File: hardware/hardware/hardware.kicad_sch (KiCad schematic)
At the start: 31 parts, among them J1 POWER, J2 SENSOR, Q1 BC547, Q2 NPN, Q3 NPN, Q4 NPN, Q5 NPN, SW1 SW_Push, SW2 SW_Push, SW5 SW_Push, U1 74HC595, U2 LM78M05_TO252, Y1 8MHz

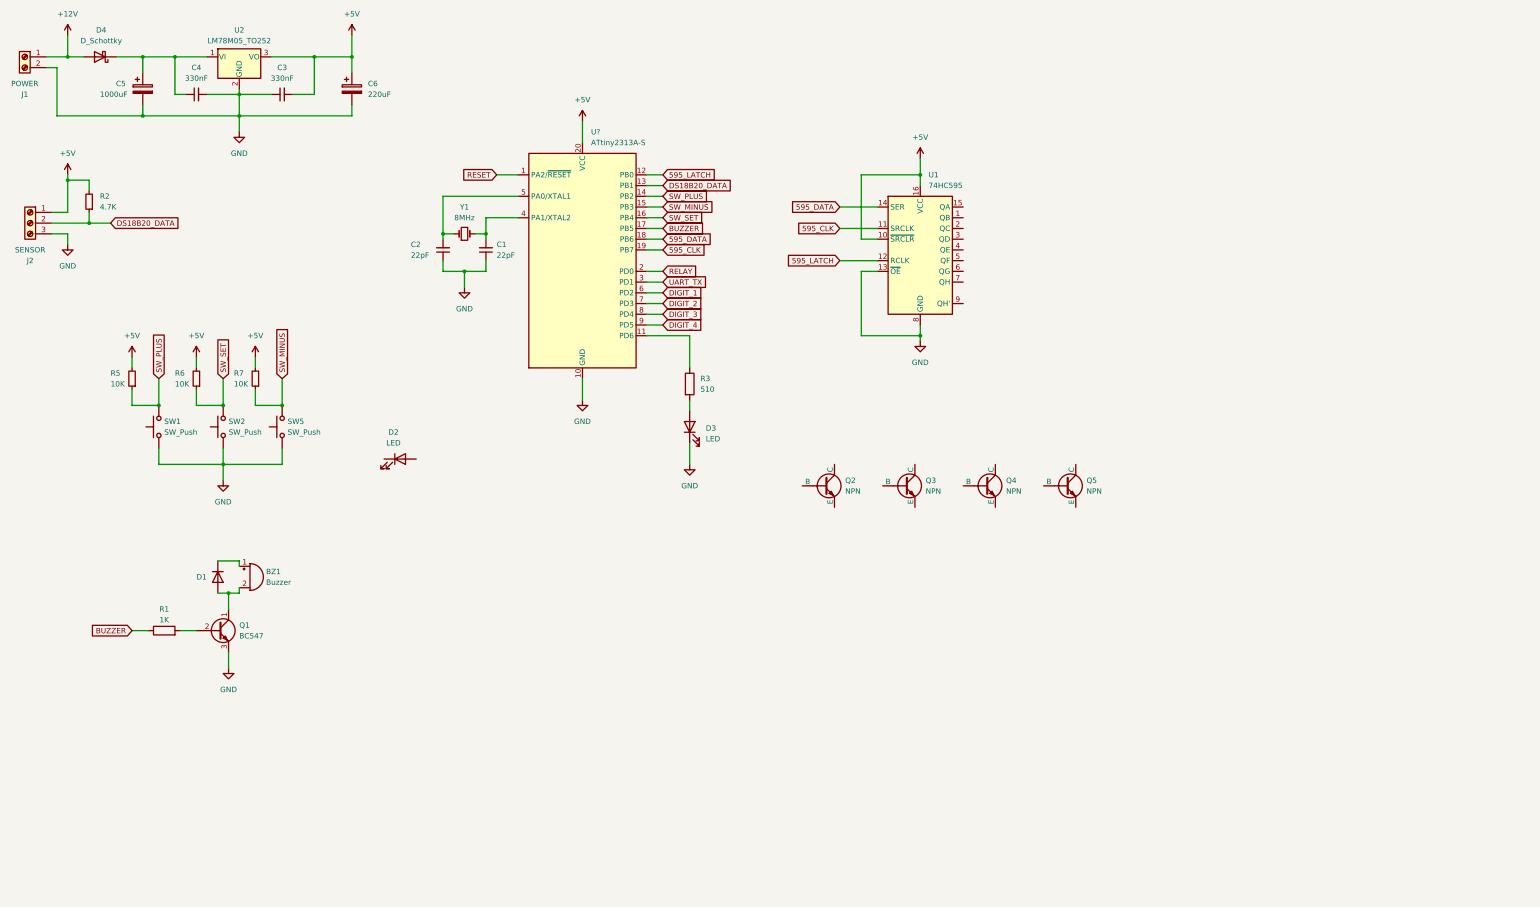
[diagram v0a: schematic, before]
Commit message: pnp
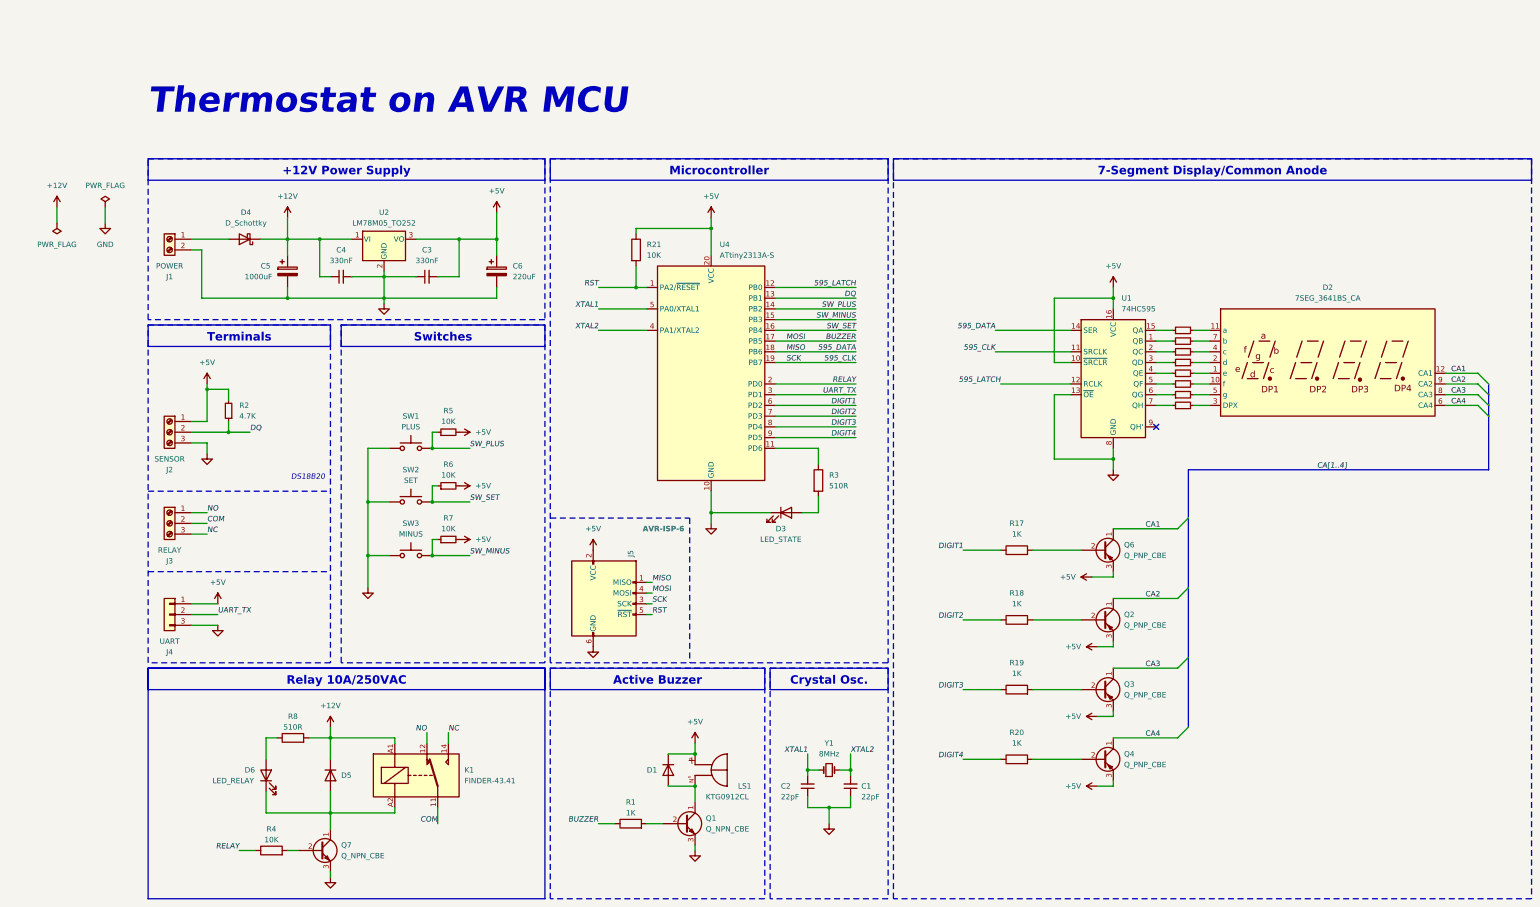
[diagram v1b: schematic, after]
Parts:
- removed BZ1: Buzzer, symbol Device:Buzzer
- removed D2: LED, symbol Device:LED
- removed Q1: BC547, Package_TO_SOT_THT:TO-92_Inline, symbol Transistor_BJT:BC547
- removed Q2, Q3, Q4, Q5: NPN, symbol Simulation_SPICE:NPN
- removed SW5: SW_Push, symbol Switch:SW_Push
- added D2: 7SEG_3641BS_CA, footprints:7SEG_3641BS, symbol components:7SEG_3641BS_CA
- added D5: D, Diode_SMD:D_SMA, symbol Device:D
- added D6: LED_RELAY, LED_SMD:LED_0805_2012Metric, symbol Device:LED
- added J3: RELAY, TerminalBlock_Phoenix:TerminalBlock_Phoenix_MPT-0,5-3-2.54_1x03_P2.54mm_Horizontal, symbol Connector:Screw_Terminal_01x03
- added J4: UART, Connector_PinHeader_2.54mm:PinHeader_1x03_P2.54mm_Vertical, symbol Connector_Generic:Conn_01x03
- added J5: AVR-ISP-6, Connector_PinHeader_2.54mm:PinHeader_2x03_P2.54mm_Vertical, symbol Connector:AVR-ISP-6
- added K1: FINDER-43.41, footprints:RELAY_FINDER-43.41, symbol components:RELAY_FINDER-43.41
- added LS1: KTG0912CL, footprints:XDCR_KTG0912CL, symbol components:KTG0912CL
- added Q1, Q7: Q_NPN_CBE, Package_TO_SOT_SMD:SOT-23, symbol Device:Q_NPN_CBE
- added Q2, Q3, Q4, Q6: Q_PNP_CBE, Package_TO_SOT_SMD:SOT-23, symbol Device:Q_PNP_CBE
- added R10, R11, R12, R13, R14, R15, R16, R9: 330R, Resistor_SMD:R_0805_2012Metric, symbol Device:R_Small
- added R17, R18, R19, R20: 1K, Resistor_SMD:R_0805_2012Metric, symbol Device:R
- added R21, R4: 10K, Resistor_SMD:R_0805_2012Metric, symbol Device:R
- added R8: 510R, Resistor_SMD:R_0805_2012Metric, symbol Device:R
- added SW3: MINUS, Button_Switch_THT:SW_PUSH_6mm_H5mm, symbol Switch:SW_Push
- C1, C2, C3, C4: footprint (none) -> Capacitor_SMD:C_0805_2012Metric
- C5: footprint (none) -> Capacitor_SMD:CP_Elec_10x10.5
- C6: footprint (none) -> Capacitor_SMD:CP_Elec_6.3x7.7
- D3: value LED -> LED_STATE; footprint (none) -> LED_SMD:LED_0805_2012Metric
- D4: footprint (none) -> Diode_SMD:D_SMA
- J1: footprint (none) -> TerminalBlock_Phoenix:TerminalBlock_Phoenix_MPT-0,5-2-2.54_1x02_P2.54mm_Horizontal
- J2: footprint (none) -> TerminalBlock_Phoenix:TerminalBlock_Phoenix_MPT-0,5-3-2.54_1x03_P2.54mm_Horizontal
- R1, R2, R5, R6, R7: footprint (none) -> Resistor_SMD:R_0805_2012Metric
- R3: value 510 -> 510R; footprint (none) -> Resistor_SMD:R_0805_2012Metric
- SW1: value SW_Push -> PLUS; footprint (none) -> Button_Switch_THT:SW_PUSH_6mm_H5mm
- SW2: value SW_Push -> SET; footprint (none) -> Button_Switch_THT:SW_PUSH_6mm_H5mm
- U1: footprint (none) -> Package_SO:SO-16_5.3x10.2mm_P1.27mm
- Y1: footprint (none) -> Crystal:Crystal_HC49-4H_Vertical
- gave numbers to parts that had none: 1
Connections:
- net +12V: now also C4.1, C5.1, D4.1 (K), U2.1 (VI), D5.1 (K), K1.A1, R8.2; no longer D4.2 (A), J1.1 (Pin_1)
- net +5V: now also D1.1 (K), J4.1 (Pin_1), J5.2 (VCC), LS1.P, Q2.3 (E), Q3.3 (E), Q4.3 (E), Q6.3 (E), R21.1
- net 595_CLK: now also J5.3 (SCK)
- net 595_DATA: now also J5.1 (MISO)
- net BUZZER: now also J5.4 (MOSI)
- net GND: now also J4.3 (Pin_3), J5.6 (GND), Q1.3 (E), Q7.3 (E), SW3.1
- net RELAY: now also R4.1
- net SW_MINUS: now also SW3.2
- net UART_TX: now also J4.2 (Pin_2)
- net at D1.2 (A): now also LS1.N, Q1.1 (C)
- net XTAL1: now reaches C2.2, U4.5 (PA0/XTAL1), Y1.1
- net at U1.1 (QB): now also R10.1
- net at U1.15 (QA): now also R9.1
- net at U1.2 (QC): now also R11.1
- net at U1.3 (QD): now also R12.1
- net at U1.4 (QE): now also R13.1
- net at U1.5 (QF): now also R14.1
- net at U1.6 (QG): now also R15.1
- net at U1.7 (QH): now also R16.1
- net XTAL2: now reaches C1.2, U4.4 (PA1/XTAL2), Y1.2
- net at R1.2: now also Q1.2 (B)
- net DIGIT_1 renamed DIGIT1
- net DIGIT1: now also R17.1
- net DIGIT_2 renamed DIGIT2
- net DIGIT2: now also R18.1
- net DIGIT_3 renamed DIGIT3
- net DIGIT3: now also R19.1
- net DIGIT_4 renamed DIGIT4
- net DIGIT4: now also R20.1
- net DS18B20_DATA renamed DQ
- net RESET renamed RST
- net RST: now also J5.5 (~{RST}), R21.2
- new net: Q2.2 (B), R18.2
- new net: Q7.2 (B), R4.2
- new net: Q6.2 (B), R17.2
- new net: D6.2 (A), R8.1
- new net: Q4.2 (B), R20.2
- new net: D2.5 (g), R15.2
- new net: D2.3 (DPX), R16.2
- new net: D2.1 (e), R13.2
- new net: D2.10 (f), R14.2
- new net: D2.11 (a), R9.2
- new net: D2.2 (d), R12.2
- new net: D2.4 (c), R11.2
- new net: D2.7 (b), R10.2
- new net: Q3.2 (B), R19.2
- new net: D5.2 (A), D6.1 (K), K1.A2, Q7.1 (C)
- new net: D4.2 (A), J1.1 (Pin_1)
- new net CA1: D2.12 (CA1), Q6.1 (C)
- new net CA2: D2.9 (CA2), Q2.1 (C)
- new net CA3: D2.8 (CA3), Q3.1 (C)
- new net CA4: D2.6 (CA4), Q4.1 (C)
- new net COM: J3.2 (Pin_2), K1.11
- new net NC: J3.3 (Pin_3), K1.14
- new net NO: J3.1 (Pin_1), K1.12
- no-connect marks 0 -> 1
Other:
- note added: "DS18B20"
- note added: "Thermostat on AVR MCU"
- moved on the sheet: C1, C2, C3, C4, C5, C6, D1, D3, D4, J1, J2, R1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
